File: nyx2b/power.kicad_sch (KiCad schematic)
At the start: 16 parts, among them J5 USB4215-03-A, U4 USBLC6-2SC6, U5 ME6211C33M5

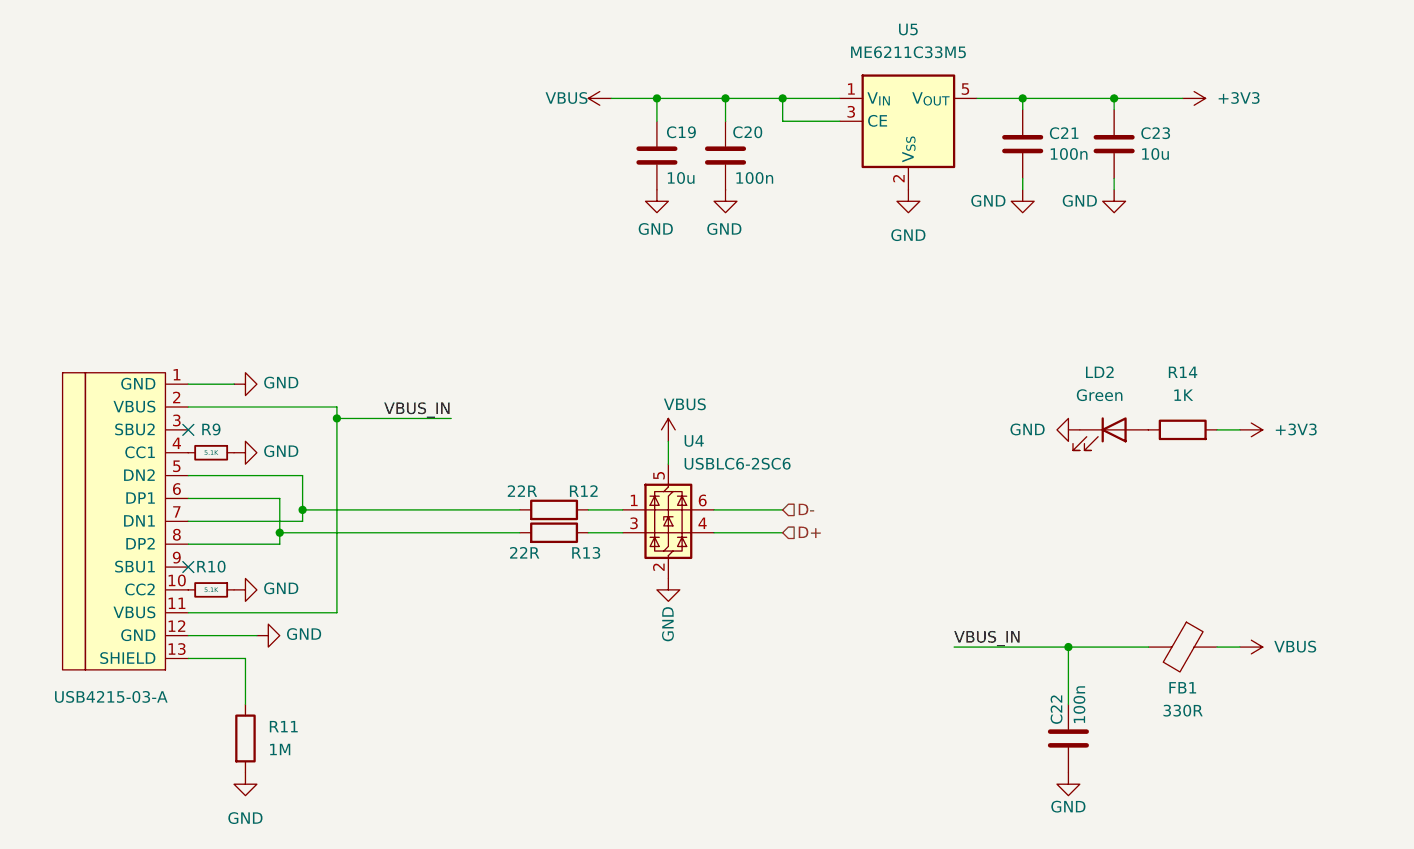
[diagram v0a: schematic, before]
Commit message: Nyx WIP
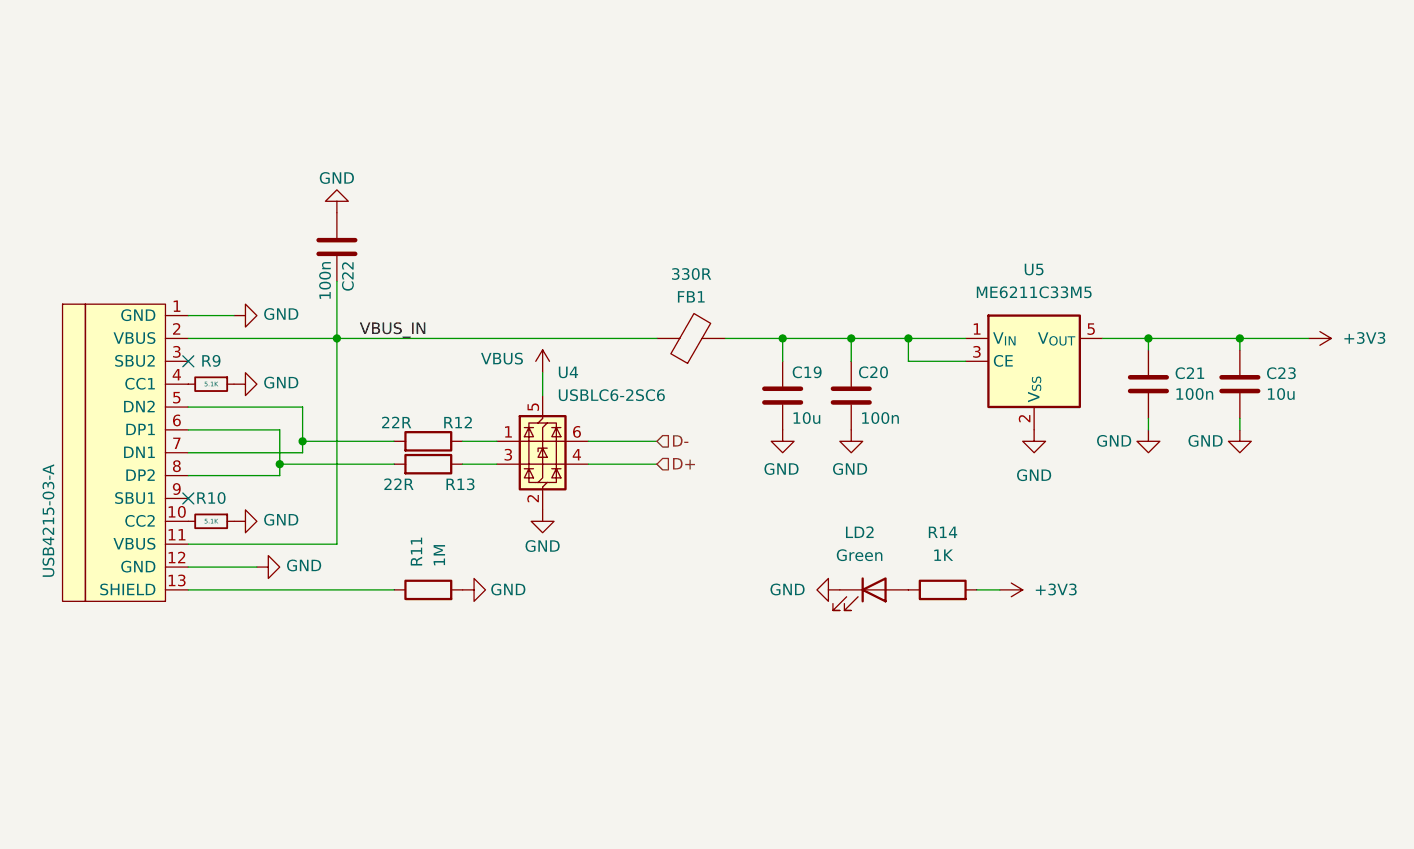
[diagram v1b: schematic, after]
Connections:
- net VBUS: no longer C19.2, C20.2, FB1.1, U5.1 (V_{IN}), U5.3 (CE)
- net VBUS_IN: now also FB1.1; no longer FB1.2
- new net: C19.2, C20.2, FB1.2, U5.1 (V_{IN}), U5.3 (CE)
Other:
- moved on the sheet: C19, C20, C21, C22, C23, FB1, LD2, R10, R11, R12, R13, R14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
